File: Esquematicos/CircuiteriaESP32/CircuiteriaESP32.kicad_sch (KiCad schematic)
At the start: 21 parts

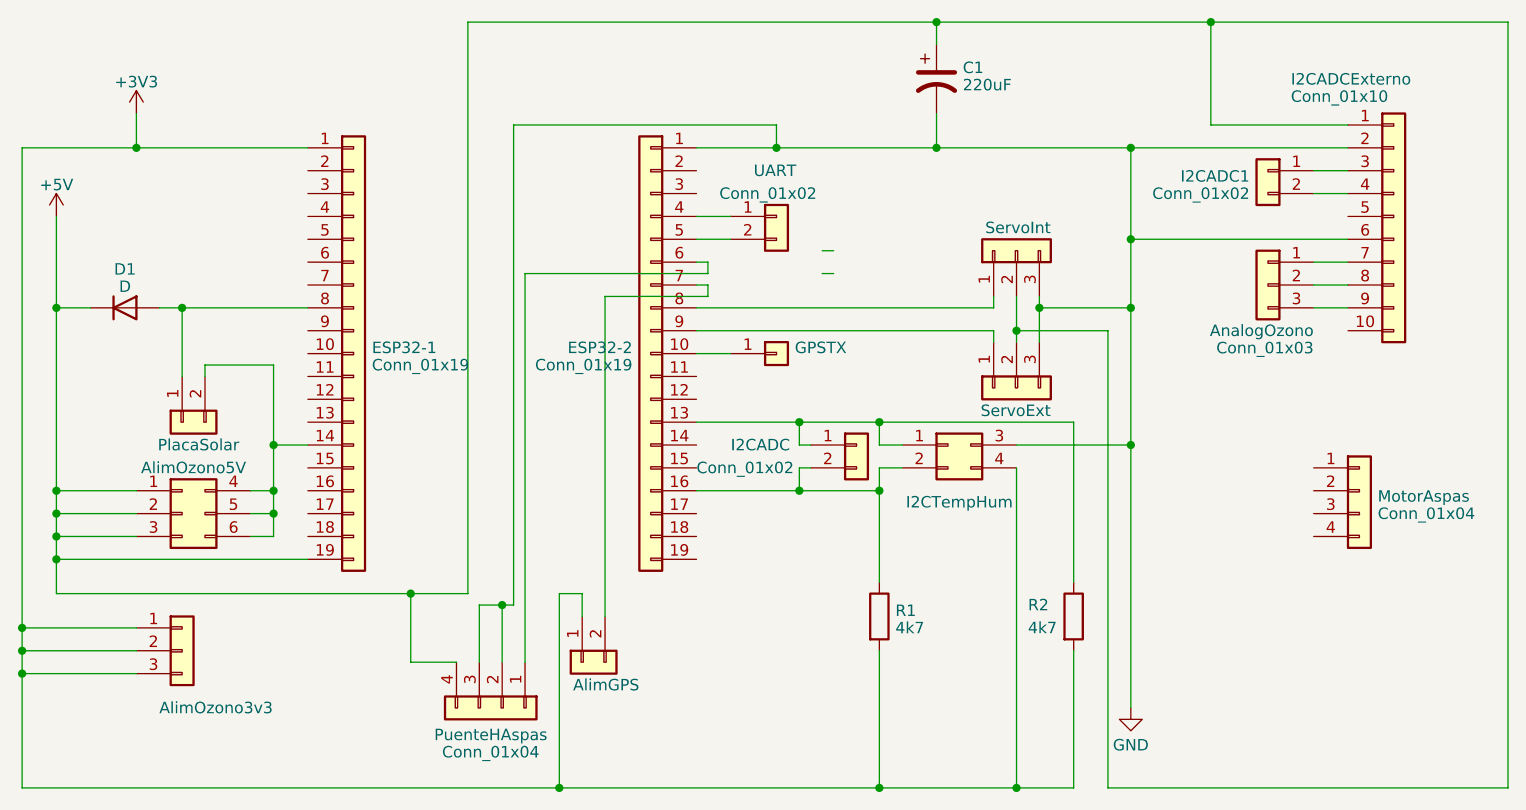
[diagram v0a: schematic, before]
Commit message: Arreglos
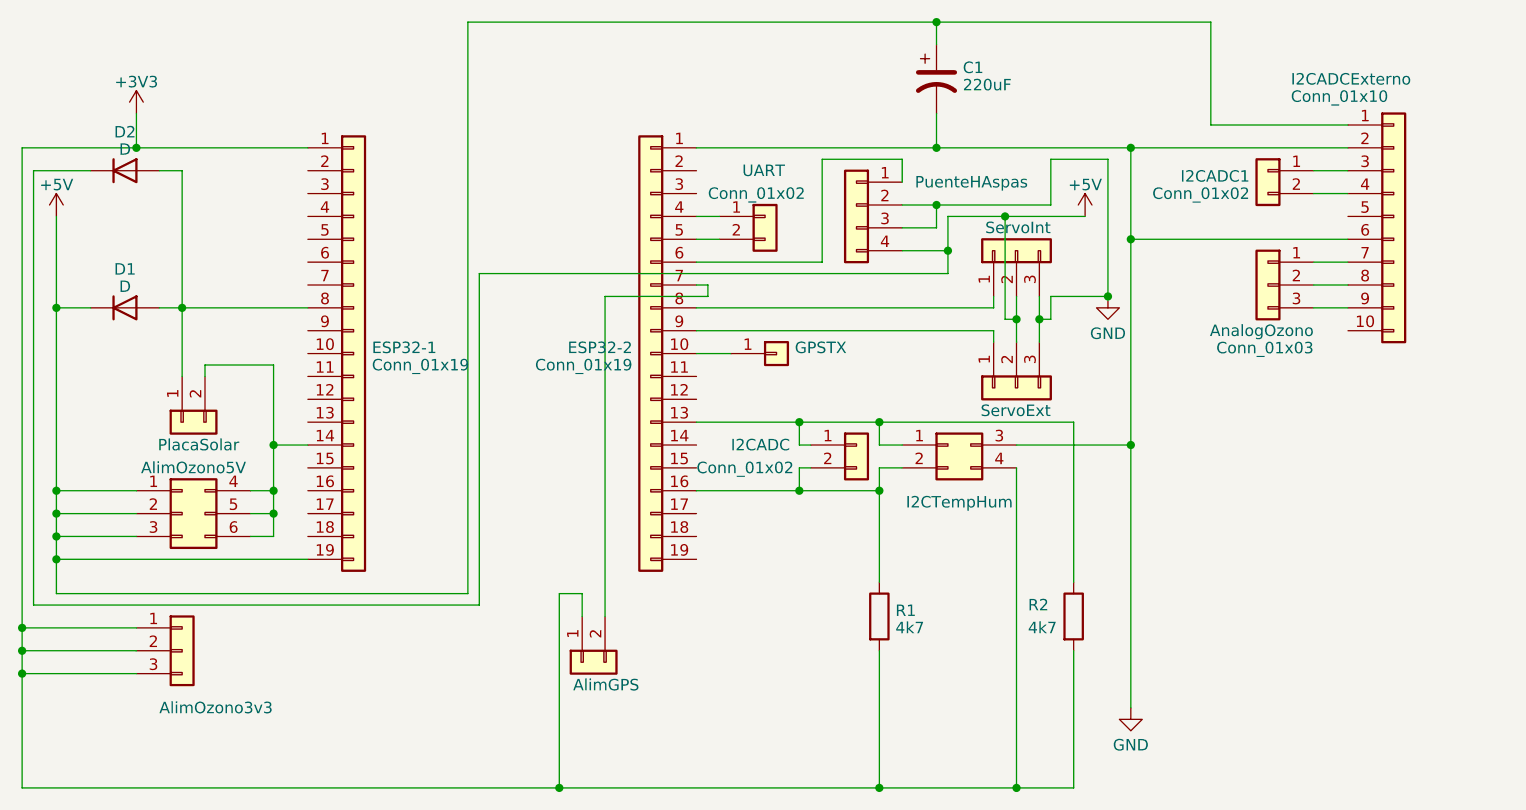
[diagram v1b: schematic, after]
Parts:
- removed MotorAspas: Conn_01x04, symbol Connector_Generic:Conn_01x04
- added D2: D, symbol Device:D
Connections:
- net +5V: now also D2.1 (K)
- net at D1.2 (A), ESP32-1.8 (Pin_8), PlacaSolar.1 (Pin_1): now also D2.2 (A)
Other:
- moved on the sheet: UART
